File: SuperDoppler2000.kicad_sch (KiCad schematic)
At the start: 8 parts

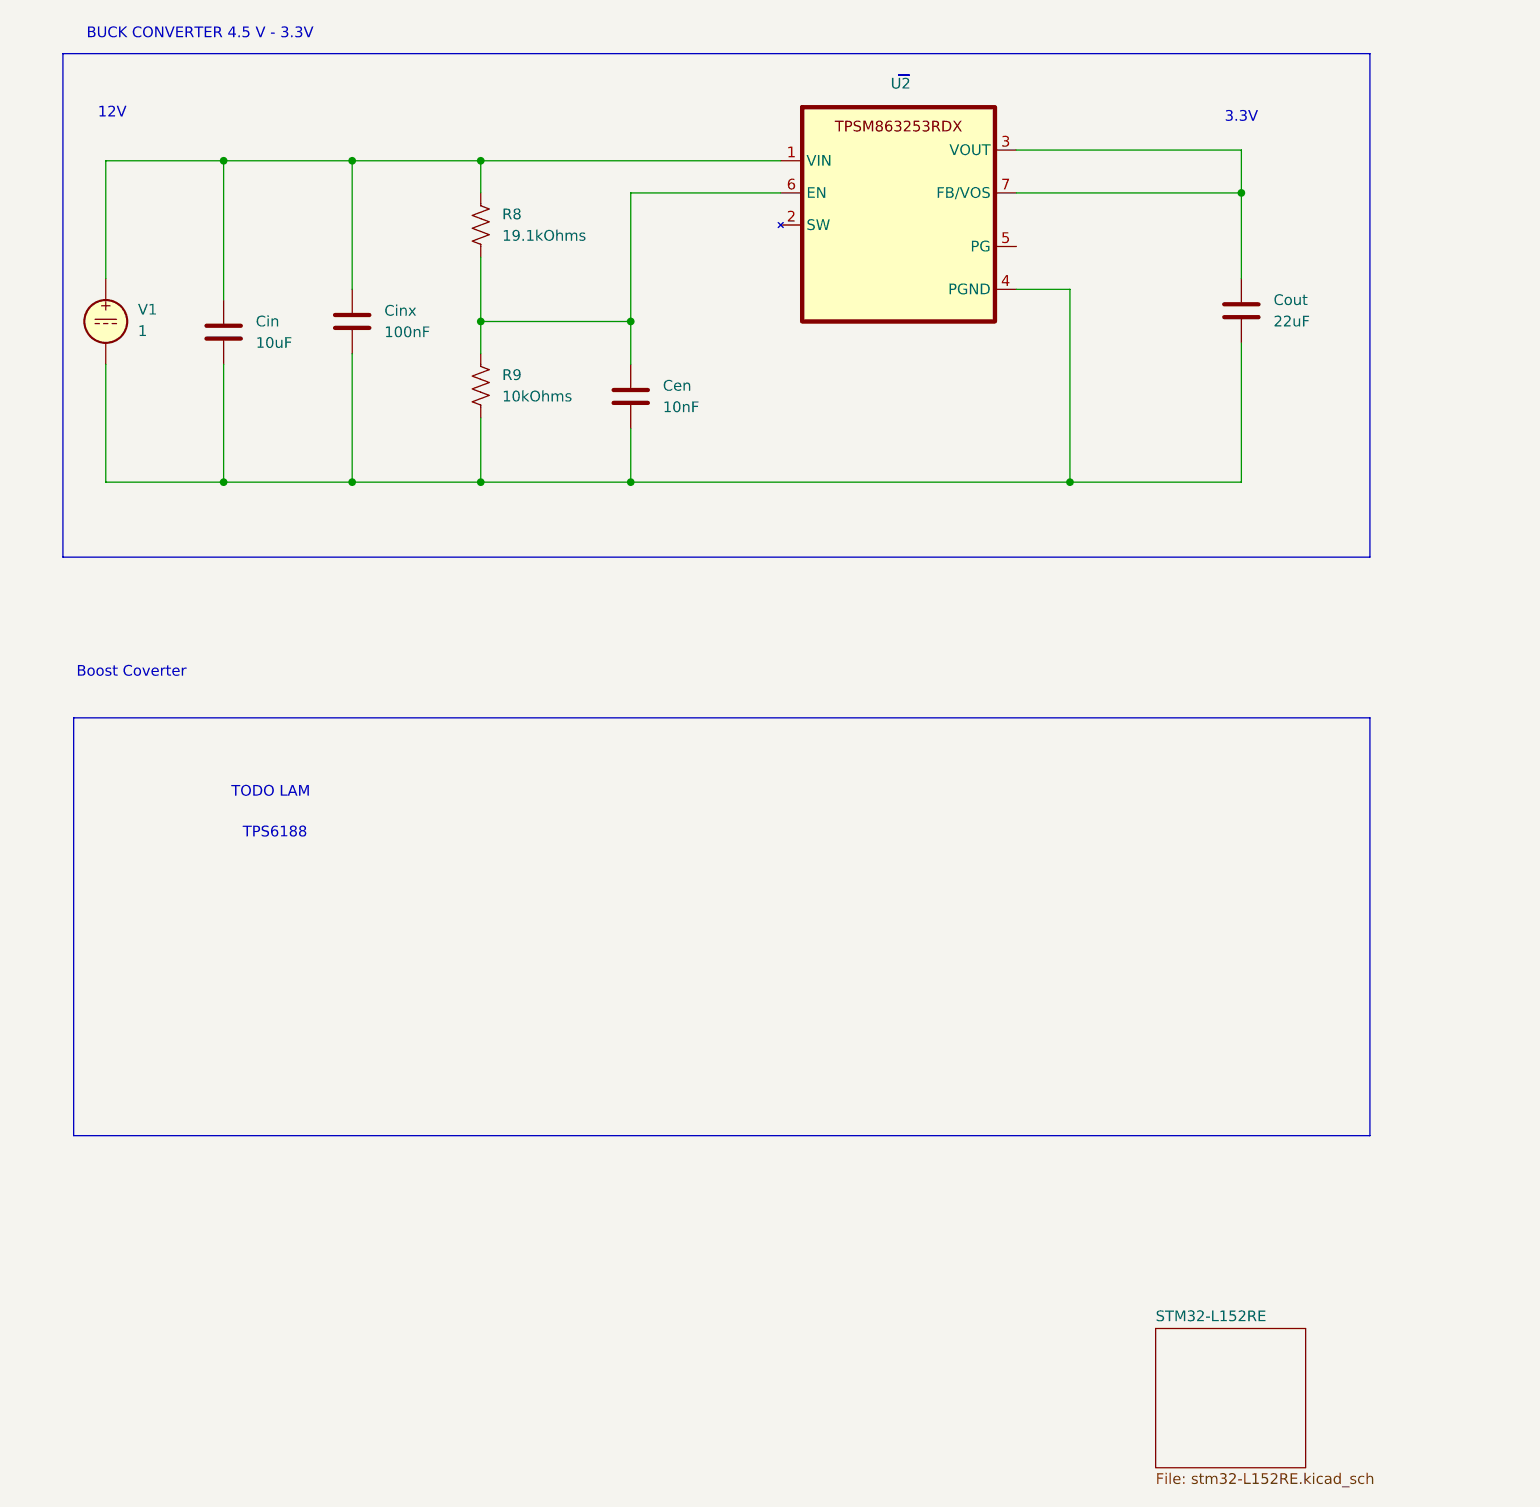
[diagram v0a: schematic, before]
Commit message: Add files via upload
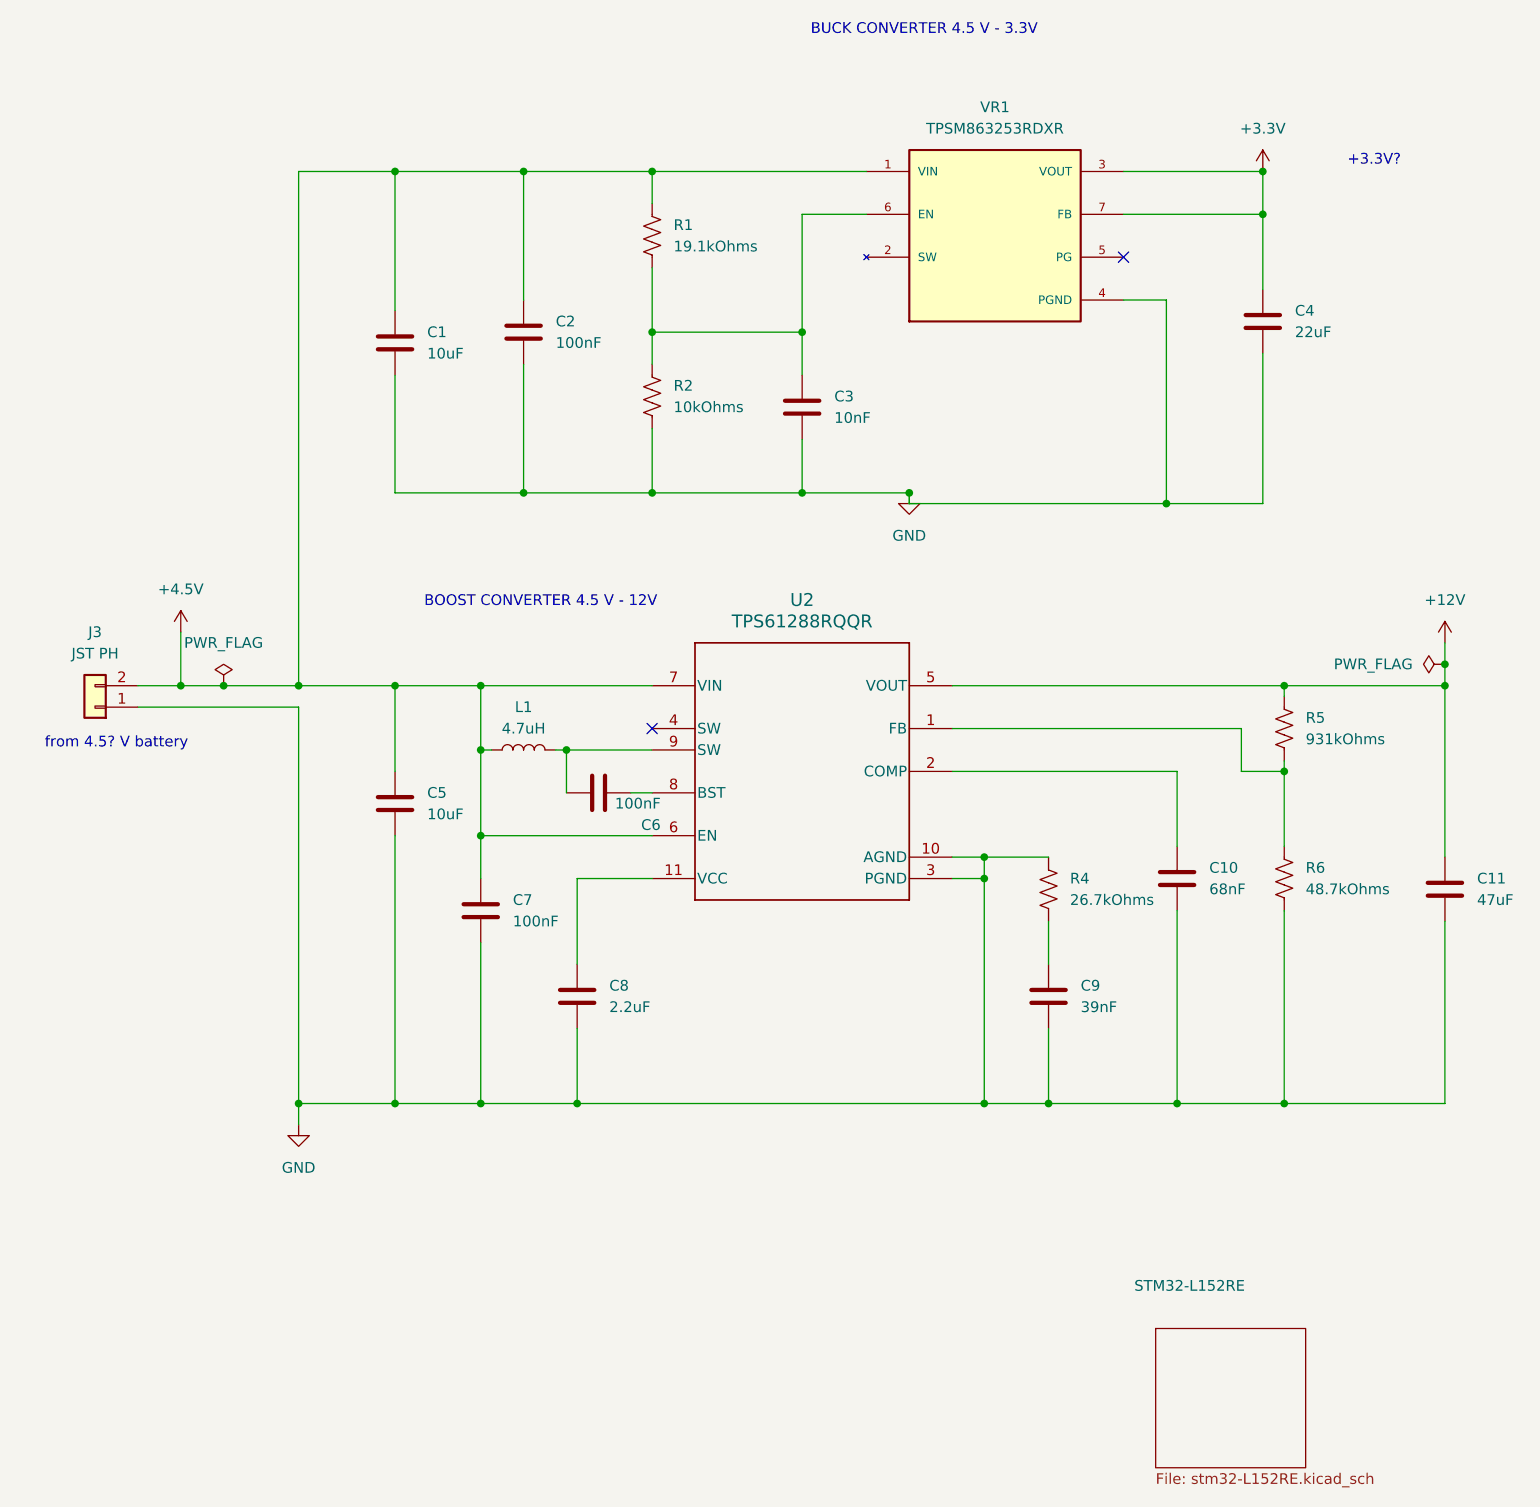
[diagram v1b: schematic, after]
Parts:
- removed U2: ~, symbol 2_Converter_DCDC:TPSM863253RDX
- removed V1: 1, symbol Simulation_SPICE:VDC
- added C10: 68nF, Capacitor_THT:C_Disc_D3.0mm_W1.6mm_P2.50mm, symbol Device:C
- added C11: 47uF, Capacitor_THT:C_Disc_D3.0mm_W1.6mm_P2.50mm, symbol Device:C
- added C5: 10uF, Capacitor_THT:C_Disc_D3.0mm_W1.6mm_P2.50mm, symbol Device:C
- added C6, C7: 100nF, Capacitor_THT:C_Disc_D3.0mm_W1.6mm_P2.50mm, symbol Device:C
- added C8: 2.2uF, Capacitor_THT:C_Disc_D3.0mm_W1.6mm_P2.50mm, symbol Device:C
- added C9: 39nF, Capacitor_THT:C_Disc_D3.0mm_W1.6mm_P2.50mm, symbol Device:C
- added J3: JST PH, Connector_JST:JST_PH_B2B-PH-K_1x02_P2.00mm_Vertical, symbol Connector_Generic:Conn_01x02
- added L1: 4.7uH, symbol Device:L
- added R4: 26.7kOhms, symbol Device:R_US
- added R5: 931kOhms, symbol Device:R_US
- added R6: 48.7kOhms, symbol Device:R_US
- added U2: TPS61288RQQR, FootprintLibrary:RQQ0011A-MFG, symbol TPS61288RQQ:TPS61288RQQR
- added VR1: TPSM863253RDXR, FootprintLibrary:VREG_TPSM863253RDXR, symbol TPSM863253RDXR:TPSM863253RDXR
- renumbered Cin to C1, Cinx to C2, Cen to C3, Cout to C4, R8 to R1, R9 to R2
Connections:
- net at C3.1, R1.2, R2.1: now also VR1.6 (EN)
- net GND: now reaches C1.2, C2.2, C3.2, C4.2, R2.2
- net GND: now also C10.2, C11.2, C5.2, C7.2, C8.2, C9.2, J3.1 (Pin_1), R4.1, R6.2, U2.10 (AGND), U2.3 (PGND), VR1.4 (PGND)
- net +4.5V: now reaches C1.1, C2.1, R1.1
- net +4.5V: now also C5.1, C7.1, J3.2 (Pin_2), L1.1, U2.6 (EN), U2.7 (VIN), VR1.1 (VIN)
- net +3.3V: now reaches C4.1
- net +3.3V: now also VR1.3 (VOUT), VR1.7 (FB)
- new net: C9.1, R4.2
- new net: C8.1, U2.11 (VCC)
- new net: R5.2, R6.1, U2.1 (FB)
- new net: C6.1, L1.2, U2.9 (SW)
- new net: C6.2, U2.8 (BST)
- new net: C10.1, U2.2 (COMP)
- new net +12V: C11.1, R5.1, U2.5 (VOUT)
- no-connect marks 0 -> 2
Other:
- note added: "+3.3V?"
- note added: "BOOST CONVERTER 4.5 V - 12V"
- note added: "from 4.5? V battery"
- note removed: "12V"
- note removed: "3.3V"
- note removed: "Boost Coverter"
- note removed: "TODO LAM"
- note removed: "TPS6188"
- moved on the sheet: C1, C2, C3, C4, R1, R2
